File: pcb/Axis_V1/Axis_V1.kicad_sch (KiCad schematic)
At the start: 40 parts, among them J1 TRANSDUCER, J10 Screw_Terminal_01x03, J11 AC_L, J12 AC_N, J2 BOILER_SSR, J3 Conn_01x03, J4 Screw_Terminal_01x02, J5 Conn_01x03, J6 BREW_SW, J7 STEAM_SW, J8 PUMP_L, J9 3WAY_L, Q1 BC847, Q2 ACST410-8BTR, Q3 ACST410-8BTR, U1 ADS1115IDGS, U2 Pico, U3 MAX31855KASA

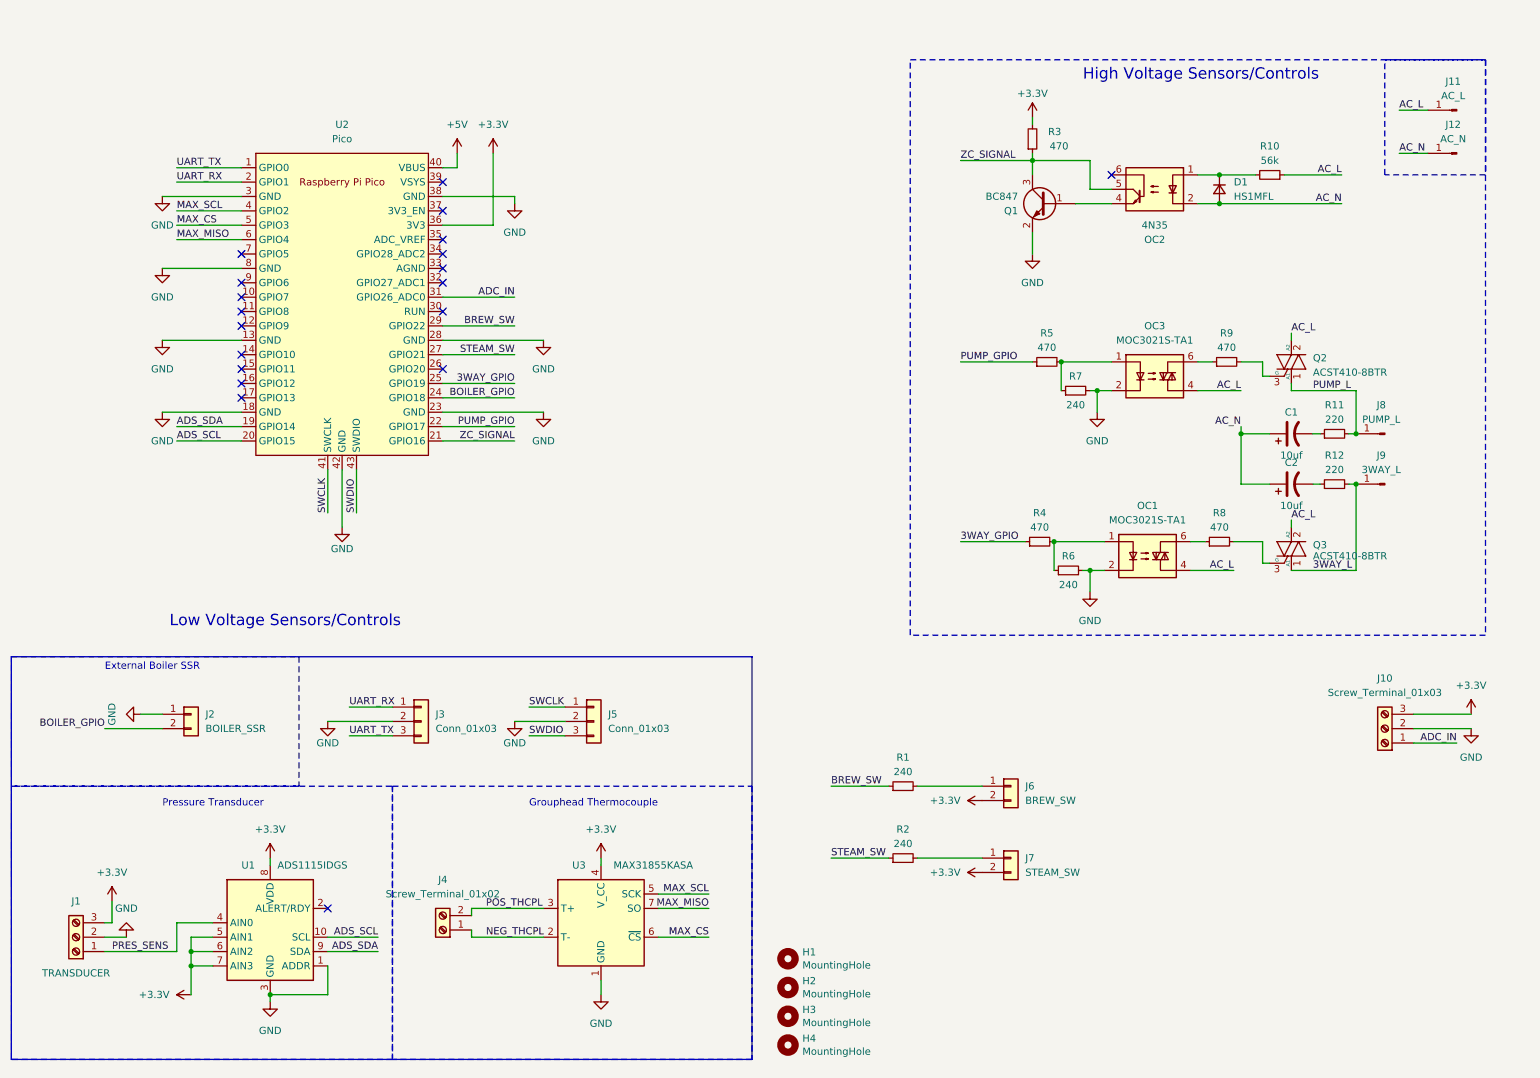
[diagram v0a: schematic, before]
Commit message: schematic updates
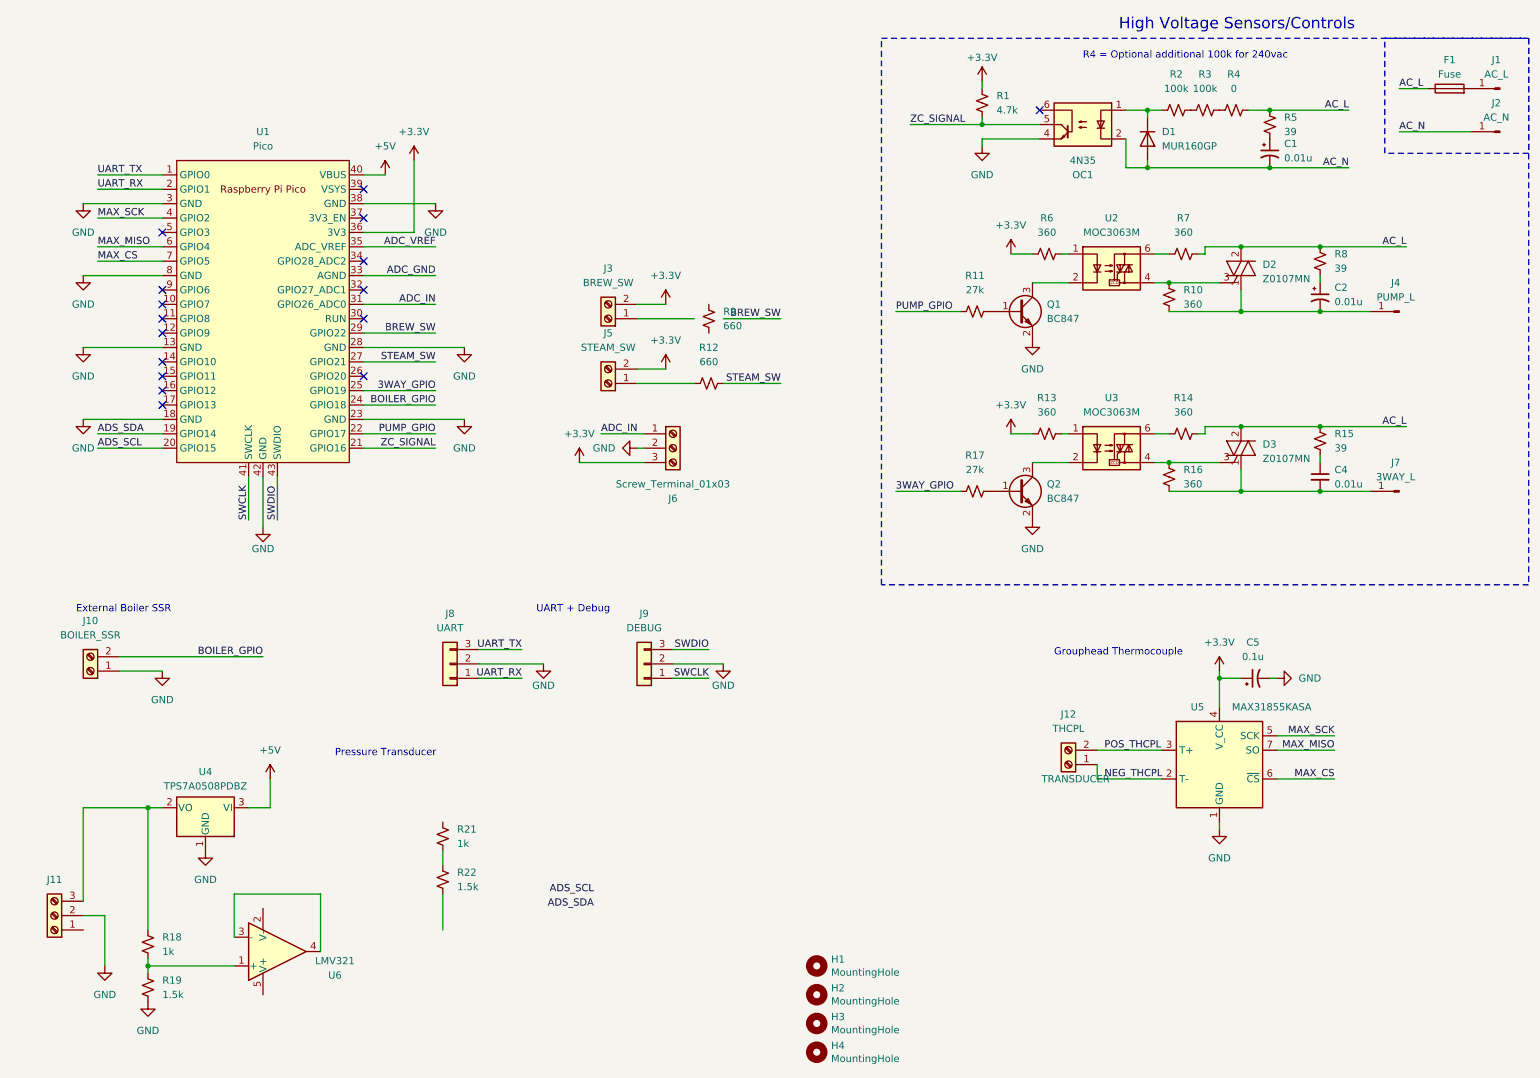
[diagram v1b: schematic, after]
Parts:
- removed C1, C2: 10uf, Capacitor_SMD:C_1206_3216Metric, symbol Device:C_Polarized_US
- removed D1: HS1MFL, Diode_SMD:D_SOD-123, symbol Device:D_Small
- removed J2: BOILER_SSR, Connector_JST:JST_PH_B2B-PH-K_1x02_P2.00mm_Vertical, symbol Connector_Generic:Conn_01x02
- removed J6: BREW_SW, Connector_JST:JST_PH_B2B-PH-K_1x02_P2.00mm_Vertical, symbol Connector_Generic:Conn_01x02
- removed J7: STEAM_SW, Connector_JST:JST_PH_B2B-PH-K_1x02_P2.00mm_Vertical, symbol Connector_Generic:Conn_01x02
- removed J8: PUMP_L, Library:Quick Disconnect, symbol Connector:Conn_01x01_Pin
- removed J9: 3WAY_L, Library:Quick Disconnect, symbol Connector:Conn_01x01_Pin
- removed OC1, OC3: MOC3021S-TA1, Package_DIP:SMDIP-6_W7.62mm, symbol Relay_SolidState:MOC3021M
- removed Q2, Q3: ACST410-8BTR, Package_TO_SOT_SMD:TO-252-2, symbol Triac_Thyristor:BT136-500
- removed R1, R2, R6, R7: 240, Resistor_SMD:R_1206_3216Metric, symbol Device:R_Small
- removed R10: 56k, Resistor_SMD:R_2512_6332Metric, symbol Device:R_Small
- removed R11, R12: 220, Resistor_SMD:R_2512_6332Metric, symbol Device:R_Small
- removed R3, R4, R5: 470, Resistor_SMD:R_1206_3216Metric, symbol Device:R_Small
- removed R8, R9: 470, Resistor_SMD:R_2512_6332Metric, symbol Device:R_Small
- removed U1: ADS1115IDGS, Package_SO:TSSOP-10_3x3mm_P0.5mm, symbol Analog_ADC:ADS1115IDGS
- added C1, C2: 0.01u, symbol Device:C_Polarized_Small_US
- added C4: 0.01u, symbol Device:C_Small
- added C5: 0.1u, symbol Device:C_Polarized_Small_US
- added D1: MUR160GP, Diode_THT:D_DO-41_SOD81_P10.16mm_Horizontal, symbol Diode:1N4007
- added D2, D3: Z0107MN, Package_TO_SOT_SMD:SOT-223, symbol Triac_Thyristor:Z0107MN
- added F1: Fuse, symbol Device:Fuse
- added J10: BOILER_SSR, TerminalBlock_MetzConnect:TerminalBlock_MetzConnect_Type101_RT01602HBWC_1x02_P5.08mm_Horizontal, symbol Connector:Screw_Terminal_01x02
- added J3: BREW_SW, TerminalBlock_MetzConnect:TerminalBlock_MetzConnect_Type101_RT01602HBWC_1x02_P5.08mm_Horizontal, symbol Connector:Screw_Terminal_01x02
- added J4: PUMP_L, Library:Quick Disconnect, symbol Connector:Conn_01x01_Pin
- added J5: STEAM_SW, TerminalBlock_MetzConnect:TerminalBlock_MetzConnect_Type101_RT01602HBWC_1x02_P5.08mm_Horizontal, symbol Connector:Screw_Terminal_01x02
- added J7: 3WAY_L, Library:Quick Disconnect, symbol Connector:Conn_01x01_Pin
- added Q2: BC847, Package_TO_SOT_SMD:SOT-23, symbol Transistor_BJT:BC847
- added R1: 4.7k, symbol Device:R_Small_US
- added R10, R13, R14, R16, R6, R7: 360, symbol Device:R_Small_US
- added R11, R17: 27k, symbol Device:R_Small_US
- added R12, R9: 660, symbol Device:R_Small_US
- added R15, R5, R8: 39, symbol Device:R_Small_US
- added R18, R21: 1k, symbol Device:R_Small_US
- added R19, R22: 1.5k, symbol Device:R_Small_US
- added R2, R3: 100k, symbol Device:R_Small_US
- added R4: 0, symbol Device:R_Small_US
- added U2, U3: MOC3063M, Package_DIP:DIP-6_W7.62mm_LongPads, symbol Relay_SolidState:MOC3063M
- added U4: TPS7A0508PDBZ, Package_TO_SOT_SMD:SOT-23, symbol Regulator_Linear:TPS7A0508PDBZ
- added U6: LMV321, symbol Amplifier_Operational:LMV321
- J12: renamed from J4; value Screw_Terminal_01x02 -> THCPL
- J8: renamed from J3; value Conn_01x03 -> UART
- J9: renamed from J5; value Conn_01x03 -> DEBUG
- renumbered J11 to J1, J1 to J11, J12 to J2, J10 to J6, OC2 to OC1, U2 to U1, U3 to U5
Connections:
- net +3.3V: now also C5.1, J3.2 (Pin_2), J5.2 (Pin_2), R1.2, R13.1, R6.2; no longer J11.3 (Pin_3)
- net +5V: now also U4.3 (VI)
- net 3WAY_GPIO: now also R17.2
- net AC_L: now also D2.2 (A2), D2.4 (A4), D3.2 (A2), D3.4 (A4), F1.1, R14.2, R15.2, R4.2, R5.2, R7.2, R8.2; no longer J1.1 (Pin_1)
- net AC_N: now also C1.2, D1.2 (A)
- net BOILER_GPIO: now also J10.2 (Pin_2)
- net GND: now also OC1.4, C5.2, J10.1 (Pin_1), Q2.2 (E), R19.2, U4.1 (GND)
- net MAX_CS: now also U1.7 (GPIO5); no longer U1.5 (GPIO3)
- net PUMP_GPIO: now also R11.2
- net STEAM_SW: now also R12.2
- net ZC_SIGNAL: now also R1.1; no longer Q1.3 (C)
- net ADC_GND: now reaches U1.33 (AGND)
- net ADC_VREF: now reaches U1.35 (ADC_VREF)
- net at OC1.1: now also D1.1 (K), R2.1
- net at Q1.1 (B): now also R11.1; no longer OC1.4
- net MAX_SCL renamed MAX_SCK
- net PRES_SENS: no longer names the net of J11.1 (Pin_1)
- new net: R18.1, R19.1, U6.1 (+)
- new net: U6.3 (-), U6.4
- new net: C4.1, R15.1
- new net: C2.2, D2.1 (A1), J4.1 (Pin_1), R10.1
- new net: C4.2, D3.1 (A1), J7.1 (Pin_1), R16.1
- new net: D3.3 (G), R16.2, U3.4
- new net: D2.3 (G), R10.2, U2.4
- new net: F1.2, J1.1 (Pin_1)
- new net: J5.1 (Pin_1), R12.1
- new net: R3.2, R4.1
- new net: R2.2, R3.1
- new net: J11.3 (Pin_3), R18.2, U4.2 (VO)
- new net: R6.1, U2.1
- new net: Q1.3 (C), U2.2
- new net: R7.1, U2.6
- new net: R21.1, R22.1
- new net: Q2.1 (B), R17.1
- new net: Q2.3 (C), U3.2
- new net: C1.1, R5.1
- new net: R14.1, U3.6
- new net: R13.2, U3.1
- new net: C2.1, R8.1
- no-connect marks 19 -> 16
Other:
- note added: "R4 = Optional additional 100k for 240vac"
- note added: "UART + Debug"
- note removed: "Low Voltage Sensors/Controls"
- moved on the sheet: H1, H2, H3, H4, J1, J11, J12, J2, J6, J8, J9, OC1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
